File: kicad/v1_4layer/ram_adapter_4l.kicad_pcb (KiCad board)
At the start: 4 copper layers, 18.3 x 41.1 mm, 5 parts, among them J1 Conn_01x16_Male, J2 Conn_01x16_Male, U1 IS61C5128AL-10KLI

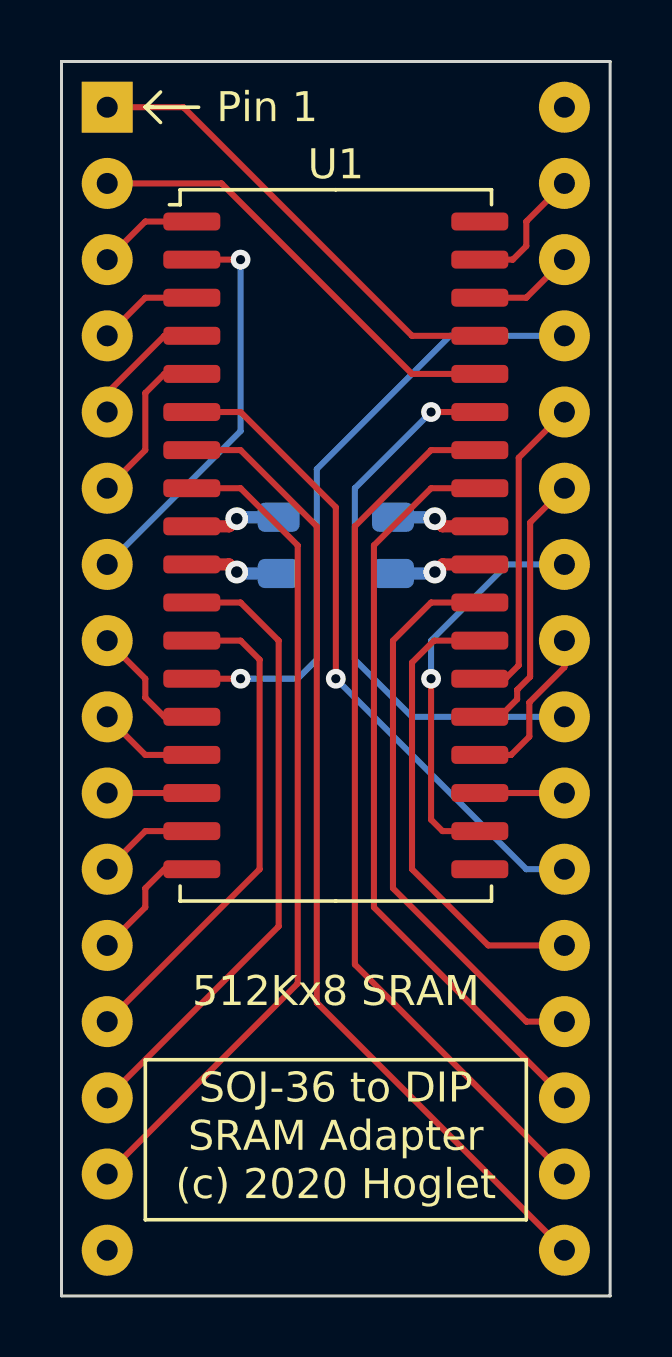
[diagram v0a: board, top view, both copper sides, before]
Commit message: Tweak thermals
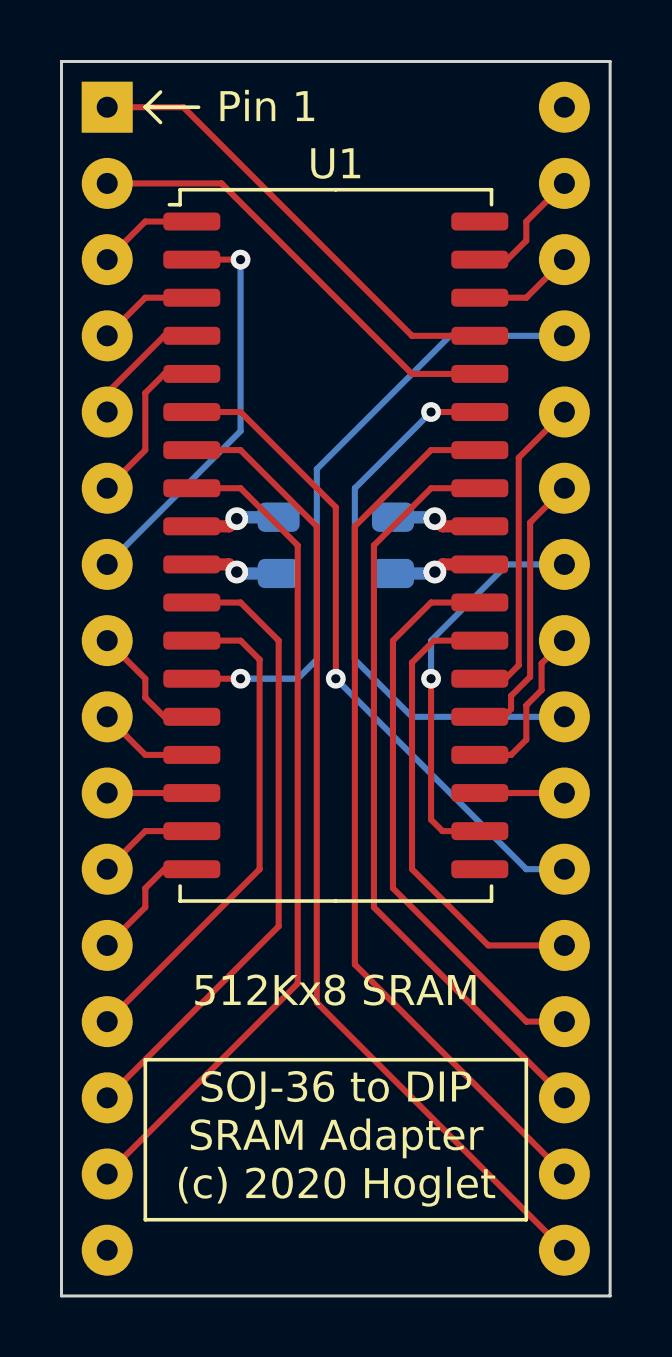
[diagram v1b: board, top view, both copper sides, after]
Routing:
- net /VCC: track 5.84 -> 15.6 mm
- net /GND: track 5.84 -> 15.6 mm
